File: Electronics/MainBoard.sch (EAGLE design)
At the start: 10 parts, among them J1 1X2-3.5MM

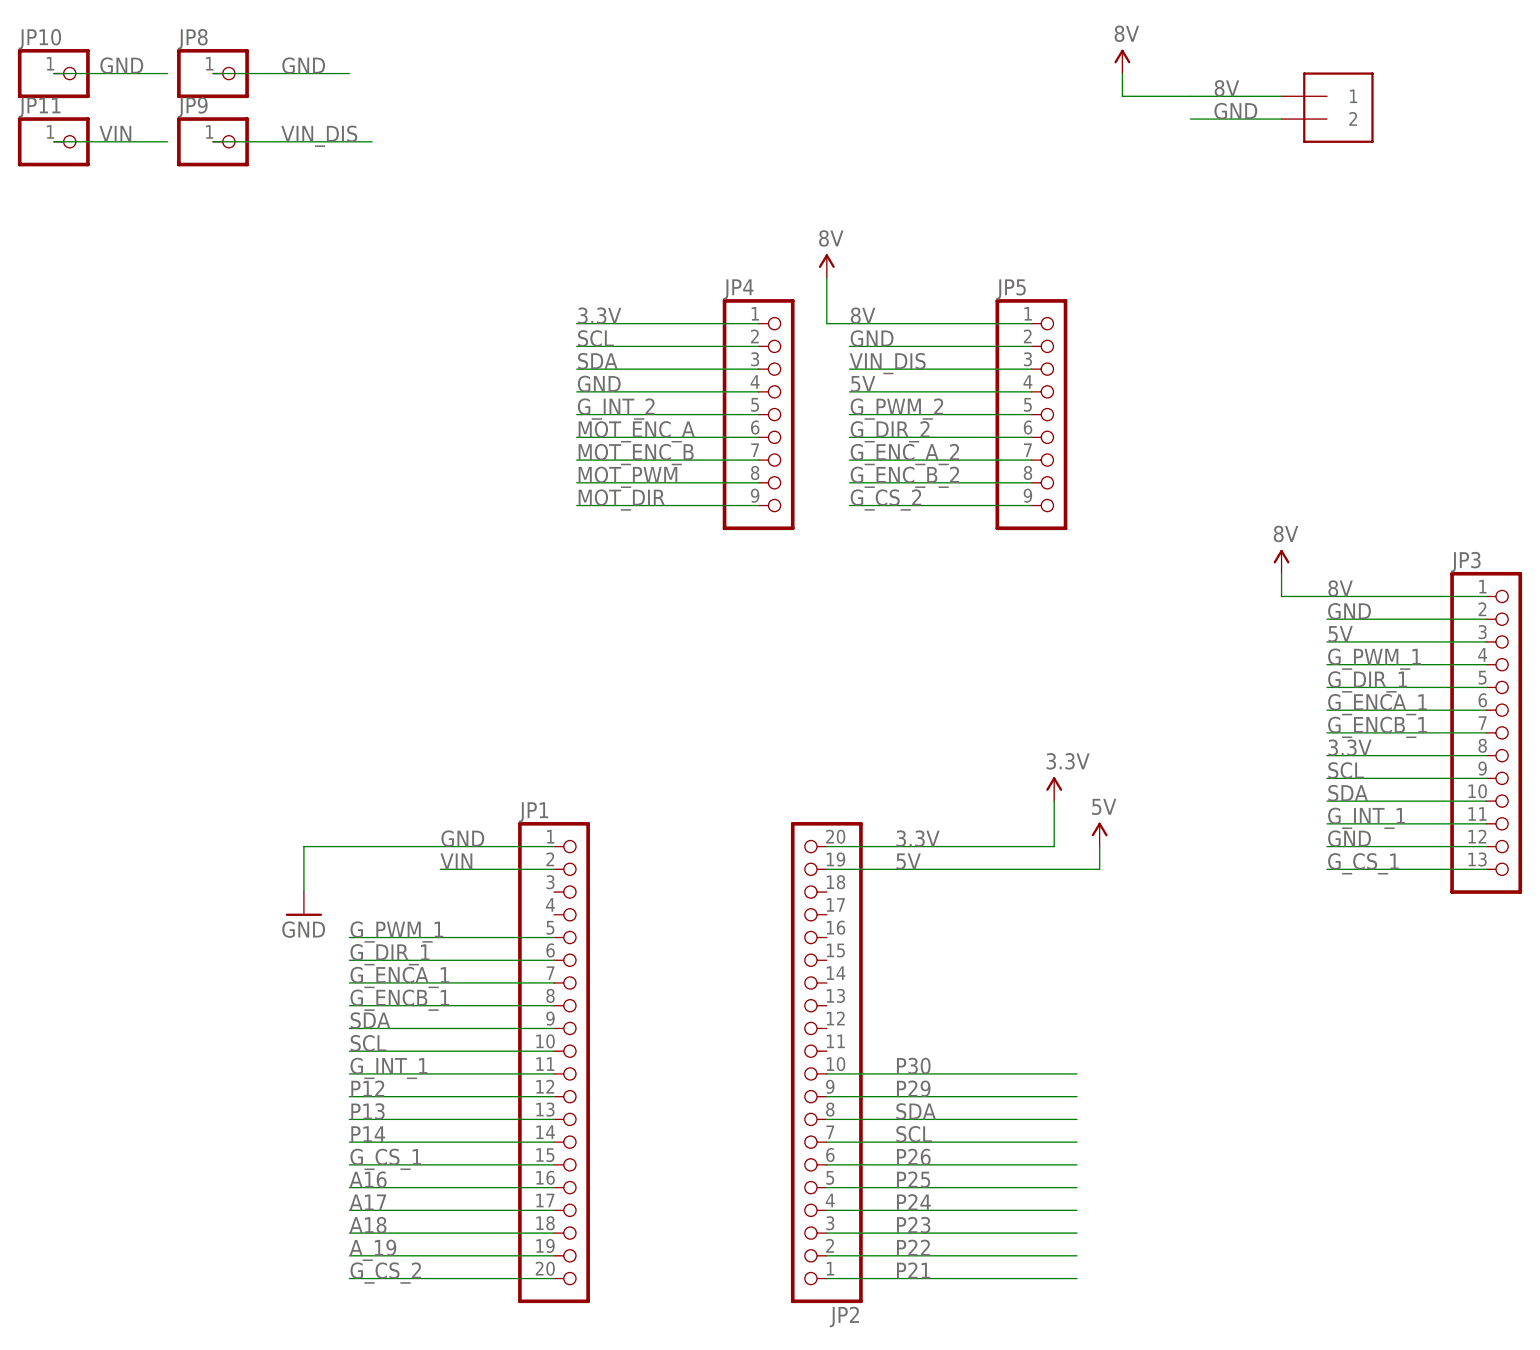
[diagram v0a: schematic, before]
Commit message: nearly done
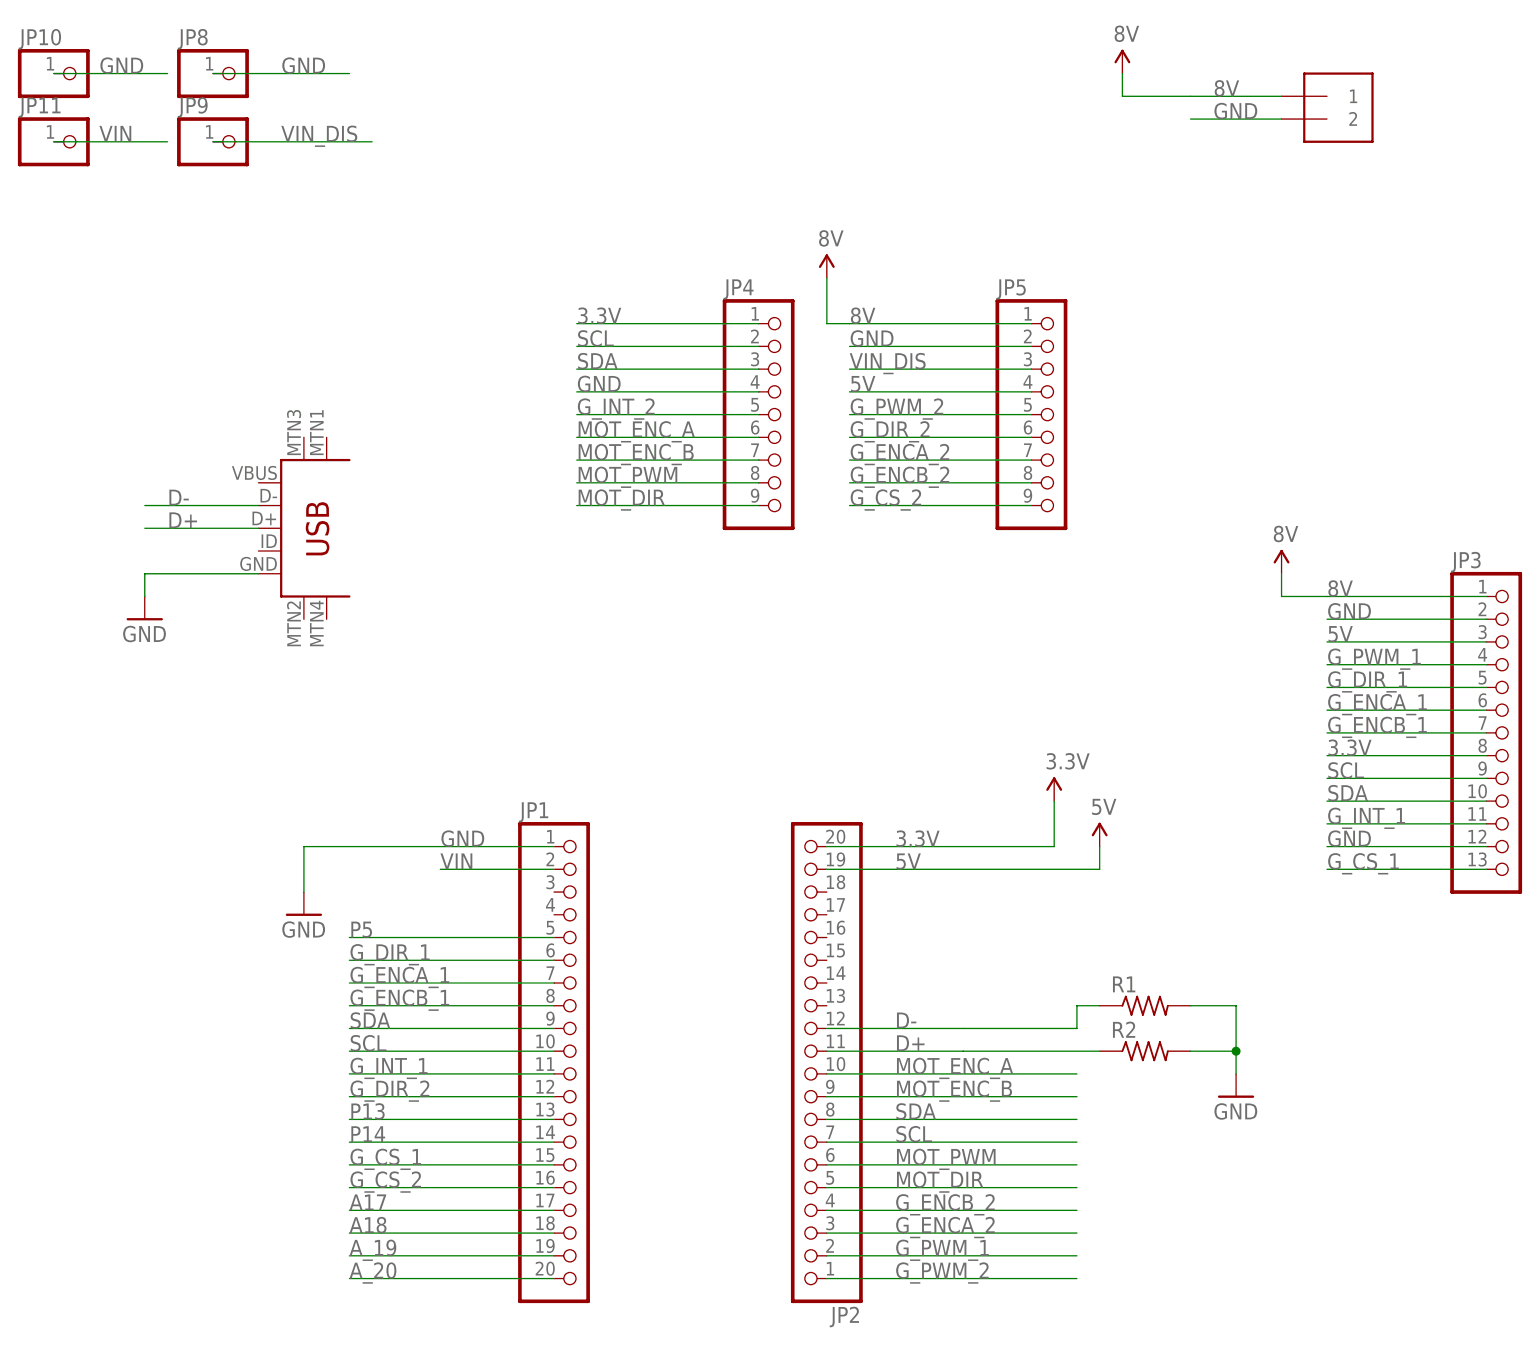
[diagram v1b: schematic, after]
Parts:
- added R1, R2: (no value), fab:RES-US1206
- added U$1: USB-MINIB-5PIN, SparkFun:USB-MINIB-5PIN
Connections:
- removed net A16: JP1.16
- removed net G_ENC_A_2: JP5.7
- removed net G_ENC_B_2: JP5.8
- removed net P12: JP1.12
- removed net P21: JP2.1
- removed net P22: JP2.2
- removed net P23: JP2.3
- removed net P24: JP2.4
- removed net P25: JP2.5
- removed net P26: JP2.6
- removed net P29: JP2.9
- removed net P30: JP2.10
- new net A_20: JP1.20
- new net D+: JP2.11, R2.1, U$1.D+
- new net D-: JP2.12, R1.1, U$1.D-
- new net G_ENCA_2: JP2.3, JP5.7
- new net G_ENCB_2: JP2.4, JP5.8
- new net P5: JP1.5
- net GND: now also R1.2, R2.2, U$1.GND
- net G_CS_2: now also JP1.16; no longer JP1.20
- net G_DIR_2: now also JP1.12
- net G_PWM_1: now also JP2.2; no longer JP1.5
- net G_PWM_2: now also JP2.1
- net MOT_DIR: now also JP2.5
- net MOT_ENC_A: now also JP2.10
- net MOT_ENC_B: now also JP2.9
- net MOT_PWM: now also JP2.6
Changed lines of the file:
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@@
 <part name="8V1" library="SparkFun" deviceset="VCC" device="" value="8V"/>
 <part name="8V2" library="SparkFun" deviceset="VCC" device="" value="8V"/>
+<part name="R1" library="fab" deviceset="RES-US" device="1206"/>
+<part name="R2" library="fab" deviceset="RES-US" device="1206"/>
+<part name="GND2" library="SparkFun" deviceset="GND" device=""/>
+<part name="U$1" library="SparkFun" deviceset="USB-MINIB" device="-5PIN"/>
+<part name="GND3" library="SparkFun" deviceset="GND" device=""/>
 </parts>
 <sheets>
@@
 <instance part="8V1" gate="1" x="78.74" y="193.04"/>
 <instance part="8V2" gate="1" x="45.72" y="170.18"/>
+<instance part="R1" gate="G$1" x="81.28" y="88.9"/>
+<instance part="R2" gate="G$1" x="81.28" y="83.82"/>
+<instance part="GND2" gate="1" x="91.44" y="78.74"/>
+<instance part="U$1" gate="G$1" x="-15.24" y="137.16"/>
+<instance part="GND3" gate="1" x="-30.48" y="132.08"/>
 </instances>
 <busses>
@@
 <wire x1="-20.32" y1="193.04" x2="-22.86" y2="193.04" width="0.1524" layer="91"/>
 </segment>
+<segment>
+<pinref part="R2" gate="G$1" pin="2"/>
+<wire x1="86.36" y1="83.82" x2="91.44" y2="83.82" width="0.1524" layer="91"/>
+<wire x1="91.44" y1="83.82" x2="91.44" y2="88.9" width="0.1524" layer="91"/>
+<pinref part="R1" gate="G$1" pin="2"/>
+<wire x1="91.44" y1="88.9" x2="86.36" y2="88.9" width="0.1524" layer="91"/>
+<pinref part="GND2" gate="1" pin="GND"/>
+<wire x1="91.44" y1="83.82" x2="91.44" y2="81.28" width="0.1524" layer="91"/>
+<junction x="91.44" y="83.82"/>
+</segment>
+<segment>
+<pinref part="U$1" gate="G$1" pin="GND"/>
+<wire x1="-17.78" y1="137.16" x2="-30.48" y2="137.16" width="0.1524" layer="91"/>
+<pinref part="GND3" gate="1" pin="GND"/>
+<wire x1="-30.48" y1="137.16" x2="-30.48" y2="134.62" width="0.1524" layer="91"/>
+</segment>
 </net>
 <net name="5V" class="0">
@@
 </segment>
 </net>
-<net name="P30" class="0">
-<segment>
-<pinref part="JP2" gate="A" pin="10"/>
-<wire x1="45.72" y1="81.28" x2="73.66" y2="81.28" width="0.1524" layer="91"/>
-<label x="53.34" y="81.28" size="1.778" layer="95"/>
-</segment>
-</net>
-<net name="P29" class="0">
-<segment>
-<pinref part="JP2" gate="A" pin="9"/>
-<wire x1="45.72" y1="78.74" x2="73.66" y2="78.74" width="0.1524" layer="91"/>
-<label x="53.34" y="78.74" size="1.778" layer="95"/>
-</segment>
-</net>
-<net name="P26" class="0">
-<segment>
-<pinref part="JP2" gate="A" pin="6"/>
-<wire x1="45.72" y1="71.12" x2="73.66" y2="71.12" width="0.1524" layer="91"/>
-<label x="53.34" y="71.12" size="1.778" layer="95"/>
-</segment>
-</net>
-<net name="P25" class="0">
-<segment>
-<pinref part="JP2" gate="A" pin="5"/>
-<wire x1="45.72" y1="68.58" x2="73.66" y2="68.58" width="0.1524" layer="91"/>
-<label x="53.34" y="68.58" size="1.778" layer="95"/>
-</segment>
-</net>
-<net name="P24" class="0">
+<net name="G_ENCB_2" class="0">
 <segment>
 <pinref part="JP2" gate="A" pin="4"/>
@@
 <label x="53.34" y="66.04" size="1.778" layer="95"/>
 </segment>
-</net>
-<net name="P22" class="0">
-<segment>
-<pinref part="JP2" gate="A" pin="2"/>
-<wire x1="45.72" y1="60.96" x2="73.66" y2="60.96" width="0.1524" layer="91"/>
-<label x="53.34" y="60.96" size="1.778" layer="95"/>
-</segment>
-</net>
-<net name="P21" class="0">
-<segment>
-<pinref part="JP2" gate="A" pin="1"/>
-<wire x1="45.72" y1="58.42" x2="73.66" y2="58.42" width="0.1524" layer="91"/>
-<label x="53.34" y="58.42" size="1.778" layer="95"/>
-</segment>
-</net>
-<net name="P12" class="0">
-<segment>
-<pinref part="JP1" gate="A" pin="12"/>
-<wire x1="15.24" y1="78.74" x2="-7.62" y2="78.74" width="0.1524" layer="91"/>
-<label x="-7.62" y="78.74" size="1.778" layer="95"/>
+<segment>
+<pinref part="JP5" gate="G$1" pin="8"/>
+<wire x1="68.58" y1="147.32" x2="48.26" y2="147.32" width="0.1524" layer="91"/>
+<label x="48.26" y="147.32" size="1.778" layer="95"/>
 </segment>
 </net>
@@
 <wire x1="15.24" y1="73.66" x2="-7.62" y2="73.66" width="0.1524" layer="91"/>
 <label x="-7.62" y="73.66" size="1.778" layer="95"/>
-</segment>
-</net>
-<net name="A16" class="0">
-<segment>
-<pinref part="JP1" gate="A" pin="16"/>
-<wire x1="15.24" y1="68.58" x2="-7.62" y2="68.58" width="0.1524" layer="91"/>
-<label x="-7.62" y="68.58" size="1.778" layer="95"/>
 </segment>
 </net>
@@
 </segment>
 </net>
-<net name="P23" class="0">
+<net name="G_ENCA_2" class="0">
 <segment>
 <pinref part="JP2" gate="A" pin="3"/>
 <wire x1="45.72" y1="63.5" x2="73.66" y2="63.5" width="0.1524" layer="91"/>
 <label x="53.34" y="63.5" size="1.778" layer="95"/>
+</segment>
+<segment>
+<pinref part="JP5" gate="G$1" pin="7"/>
+<wire x1="68.58" y1="149.86" x2="48.26" y2="149.86" width="0.1524" layer="91"/>
+<label x="48.26" y="149.86" size="1.778" layer="95"/>
 </segment>
 </net>
@@
 </segment>
 <segment>
-<pinref part="JP1" gate="A" pin="5"/>
-<wire x1="15.24" y1="96.52" x2="-7.62" y2="96.52" width="0.1524" layer="91"/>
-<label x="-7.62" y="96.52" size="1.778" layer="95"/>
+<pinref part="JP2" gate="A" pin="2"/>
+<wire x1="45.72" y1="60.96" x2="73.66" y2="60.96" width="0.1524" layer="91"/>
+<label x="53.34" y="60.96" size="1.778" layer="95"/>
 </segment>
 </net>
@@
 <label x="48.26" y="154.94" size="1.778" layer="95"/>
 </segment>
+<segment>
+<pinref part="JP2" gate="A" pin="1"/>
+<wire x1="45.72" y1="58.42" x2="73.66" y2="58.42" width="0.1524" layer="91"/>
+<label x="53.34" y="58.42" size="1.778" layer="95"/>
+</segment>
 </net>
 <net name="G_DIR_2" class="0">
@@
 <label x="48.26" y="152.4" size="1.778" layer="95"/>
 </segment>
-</net>
-<net name="G_ENC_A_2" class="0">
-<segment>
-<pinref part="JP5" gate="G$1" pin="7"/>
-<wire x1="68.58" y1="149.86" x2="48.26" y2="149.86" width="0.1524" layer="91"/>
-<label x="48.26" y="149.86" size="1.778" layer="95"/>
-</segment>
-</net>
-<net name="G_ENC_B_2" class="0">
-<segment>
-<pinref part="JP5" gate="G$1" pin="8"/>
-<wire x1="68.58" y1="147.32" x2="48.26" y2="147.32" width="0.1524" layer="91"/>
-<label x="48.26" y="147.32" size="1.778" layer="95"/>
+<segment>
+<pinref part="JP1" gate="A" pin="12"/>
+<wire x1="15.24" y1="78.74" x2="-7.62" y2="78.74" width="0.1524" layer="91"/>
+<label x="-7.62" y="78.74" size="1.778" layer="95"/>
 </segment>
 </net>
@@
 <label x="17.78" y="149.86" size="1.778" layer="95"/>
 </segment>
+<segment>
+<pinref part="JP2" gate="A" pin="9"/>
+<wire x1="45.72" y1="78.74" x2="73.66" y2="78.74" width="0.1524" layer="91"/>
+<label x="53.34" y="78.74" size="1.778" layer="95"/>
+</segment>
 </net>
 <net name="MOT_PWM" class="0">
@@
 <label x="17.78" y="147.32" size="1.778" layer="95"/>
 </segment>
+<segment>
+<pinref part="JP2" gate="A" pin="6"/>
+<wire x1="45.72" y1="71.12" x2="73.66" y2="71.12" width="0.1524" layer="91"/>
+<label x="53.34" y="71.12" size="1.778" layer="95"/>
+</segment>
 </net>
 <net name="MOT_DIR" class="0">
@@
 <wire x1="38.1" y1="144.78" x2="17.78" y2="144.78" width="0.1524" layer="91"/>
 <label x="17.78" y="144.78" size="1.778" layer="95"/>
+</segment>
+<segment>
+<pinref part="JP2" gate="A" pin="5"/>
+<wire x1="45.72" y1="68.58" x2="73.66" y2="68.58" width="0.1524" layer="91"/>
+<label x="53.34" y="68.58" size="1.778" layer="95"/>
 </segment>
 </net>
@@
 </segment>
 <segment>
-<pinref part="JP1" gate="A" pin="20"/>
-<wire x1="15.24" y1="58.42" x2="-7.62" y2="58.42" width="0.1524" layer="91"/>
-<label x="-7.62" y="58.42" size="1.778" layer="95"/>
+<pinref part="JP1" gate="A" pin="16"/>
+<wire x1="15.24" y1="68.58" x2="-7.62" y2="68.58" width="0.1524" layer="91"/>
+<label x="-7.62" y="68.58" size="1.778" layer="95"/>
 </segment>
 </net>
@@
 <wire x1="38.1" y1="152.4" x2="17.78" y2="152.4" width="0.1524" layer="91"/>
 <label x="17.78" y="152.4" size="1.778" layer="95"/>
+</segment>
+<segment>
+<pinref part="JP2" gate="A" pin="10"/>
+<wire x1="45.72" y1="81.28" x2="73.66" y2="81.28" width="0.1524" layer="91"/>
+<label x="53.34" y="81.28" size="1.778" layer="95"/>
 </segment>
 </net>
@@
 </segment>
 </net>
+<net name="P5" class="0">
+<segment>
+<pinref part="JP1" gate="A" pin="5"/>
+<wire x1="15.24" y1="96.52" x2="-7.62" y2="96.52" width="0.1524" layer="91"/>
+<label x="-7.62" y="96.52" size="1.778" layer="95"/>
+</segment>
+</net>
+<net name="A_20" class="0">
+<segment>
+<pinref part="JP1" gate="A" pin="20"/>
+<wire x1="15.24" y1="58.42" x2="-7.62" y2="58.42" width="0.1524" layer="91"/>
+<label x="-7.62" y="58.42" size="1.778" layer="95"/>
+</segment>
+</net>
+<net name="D+" class="0">
+<segment>
+<pinref part="JP2" gate="A" pin="11"/>
+<wire x1="45.72" y1="83.82" x2="60.96" y2="83.82" width="0.1524" layer="91"/>
+<label x="53.34" y="83.82" size="1.778" layer="95"/>
+<pinref part="R2" gate="G$1" pin="1"/>
+<wire x1="60.96" y1="83.82" x2="76.2" y2="83.82" width="0.1524" layer="91"/>
+</segment>
+<segment>
+<pinref part="U$1" gate="G$1" pin="D+"/>
+<wire x1="-17.78" y1="142.24" x2="-30.48" y2="142.24" width="0.1524" layer="91"/>
+<label x="-27.94" y="142.24" size="1.778" layer="95"/>
+</segment>
+</net>
+<net name="D-" class="0">
+<segment>
+<pinref part="JP2" gate="A" pin="12"/>
+<wire x1="45.72" y1="86.36" x2="60.96" y2="86.36" width="0.1524" layer="91"/>
+<label x="53.34" y="86.36" size="1.778" layer="95"/>
+<wire x1="60.96" y1="86.36" x2="73.66" y2="86.36" width="0.1524" layer="91"/>
+<wire x1="73.66" y1="86.36" x2="73.66" y2="88.9" width="0.1524" layer="91"/>
+<pinref part="R1" gate="G$1" pin="1"/>
+<wire x1="73.66" y1="88.9" x2="76.2" y2="88.9" width="0.1524" layer="91"/>
+</segment>
+<segment>
+<pinref part="U$1" gate="G$1" pin="D-"/>
+<wire x1="-17.78" y1="144.78" x2="-30.48" y2="144.78" width="0.1524" layer="91"/>
+<label x="-27.94" y="144.78" size="1.778" layer="95"/>
+</segment>
+</net>
